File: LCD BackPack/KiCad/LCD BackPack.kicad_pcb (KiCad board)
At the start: 2 copper layers, 45.7 x 22.9 mm, 6 parts, among them J1 8-pin_female_header_LCD_inter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, J2 Conn_01x01_Female, J3 Conn_01x01_Female, U1 LCD_HD44780

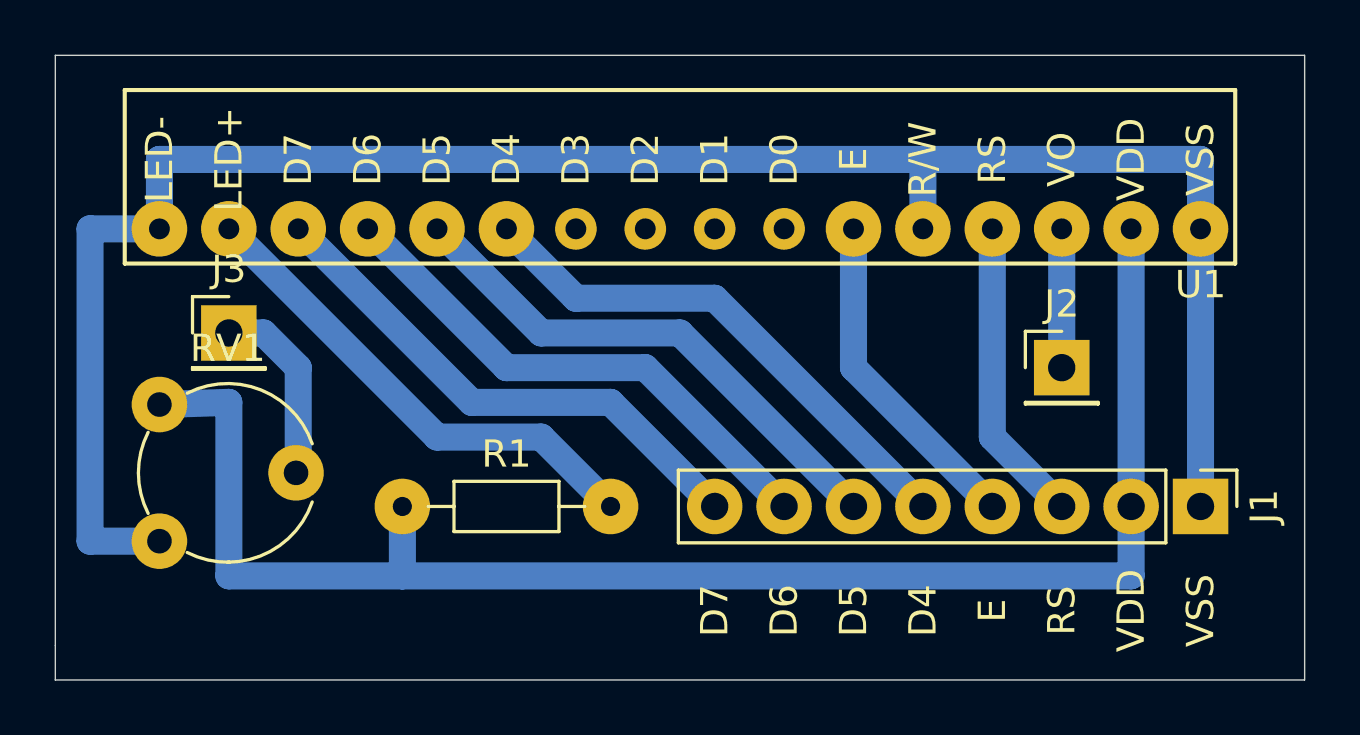
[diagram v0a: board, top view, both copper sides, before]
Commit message: copper pour
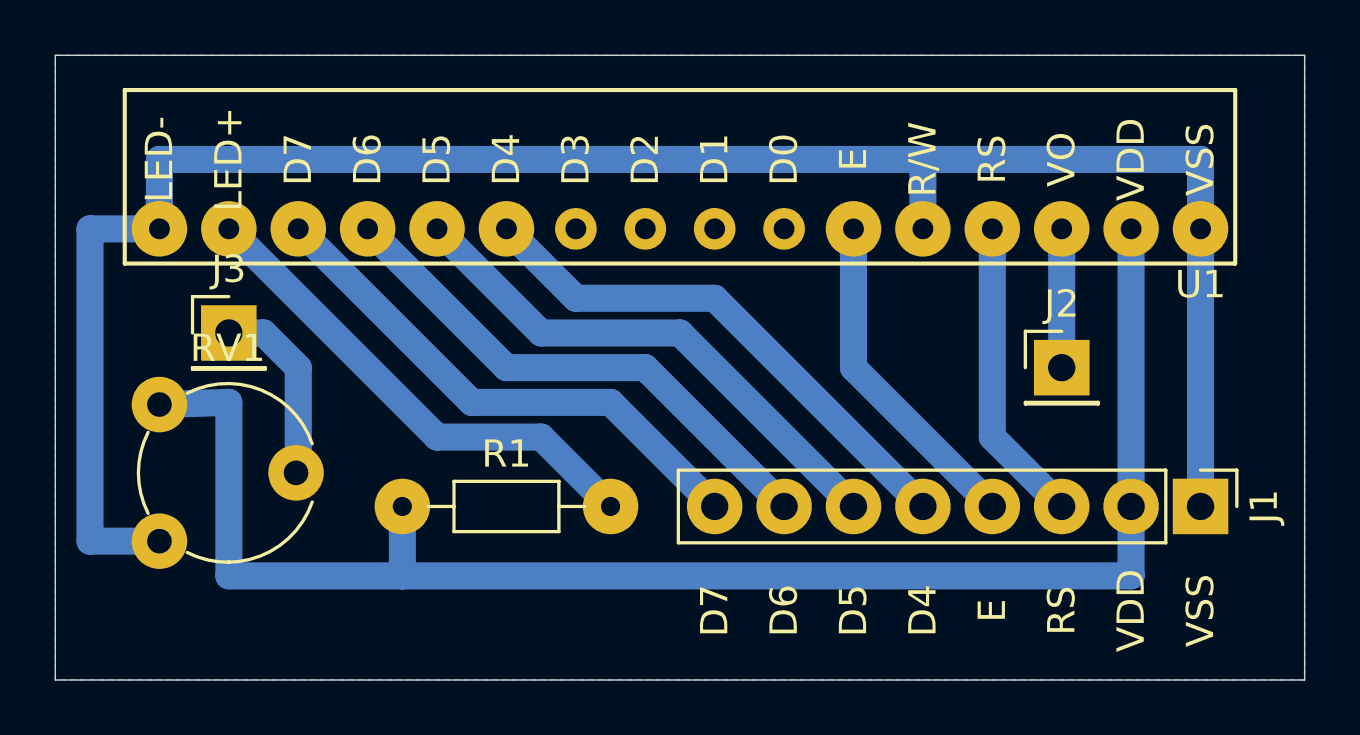
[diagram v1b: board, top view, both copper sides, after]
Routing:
- added copper zone on B.Cu, net Net-(J1-Pad1)
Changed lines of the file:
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@@
   (segment (start 132.08 100.33) (end 133.35 101.6) (width 0.9906) (layer B.Cu) (net 14))
   (segment (start 133.35 101.6) (end 133.35 105.41) (width 0.9906) (layer B.Cu) (net 14))
+  (zone (net 8) (net_name "Net-(J1-Pad1)") (layer B.Cu) (hatch edge 0.508)
+    (connect_pads (clearance 0.508))
+    (min_thickness 0.254)
+    (fill yes (arc_segments 32) (thermal_gap 0.508) (thermal_bridge_width 0.508))
+    (polygon
+      (pts
+        (xy 170.18 113.03) (xy 124.46 113.03) (xy 124.46 90.17) (xy 170.18 90.17)
+      )
+    )
+  )
 )

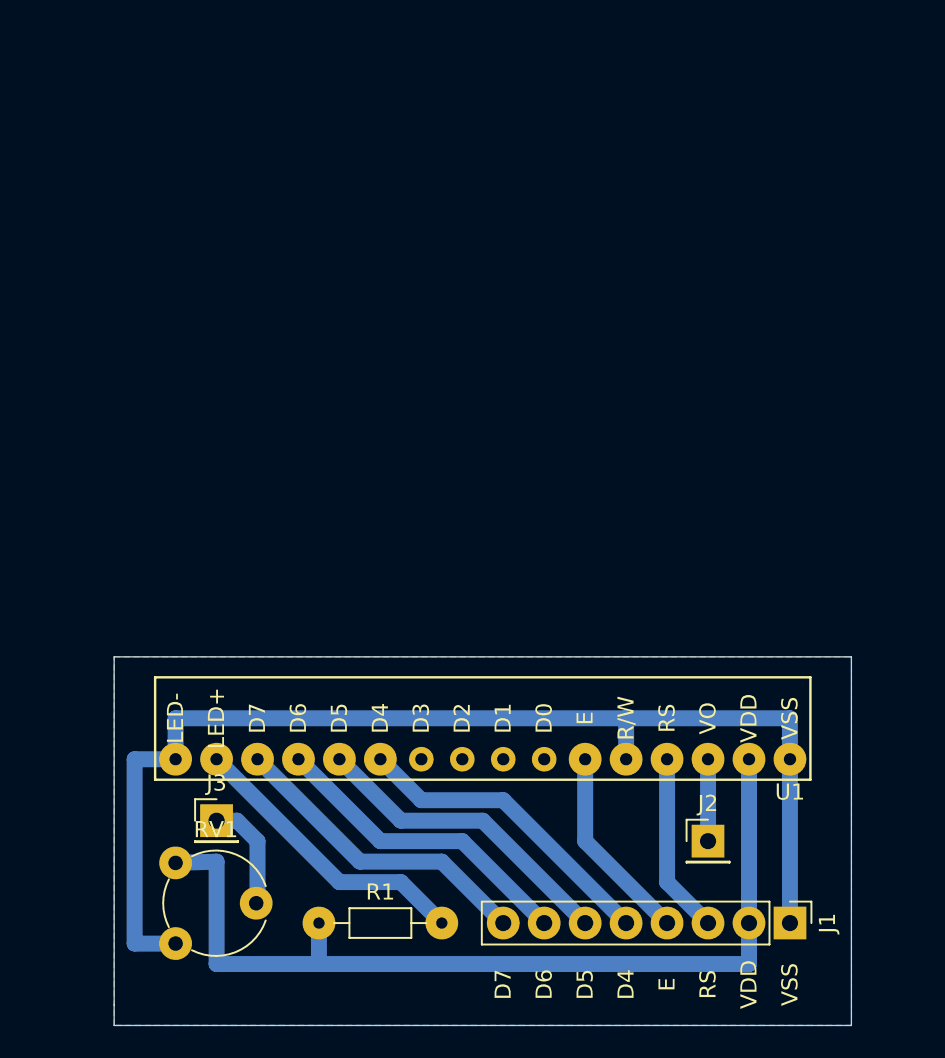
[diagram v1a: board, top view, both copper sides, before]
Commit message: new layout
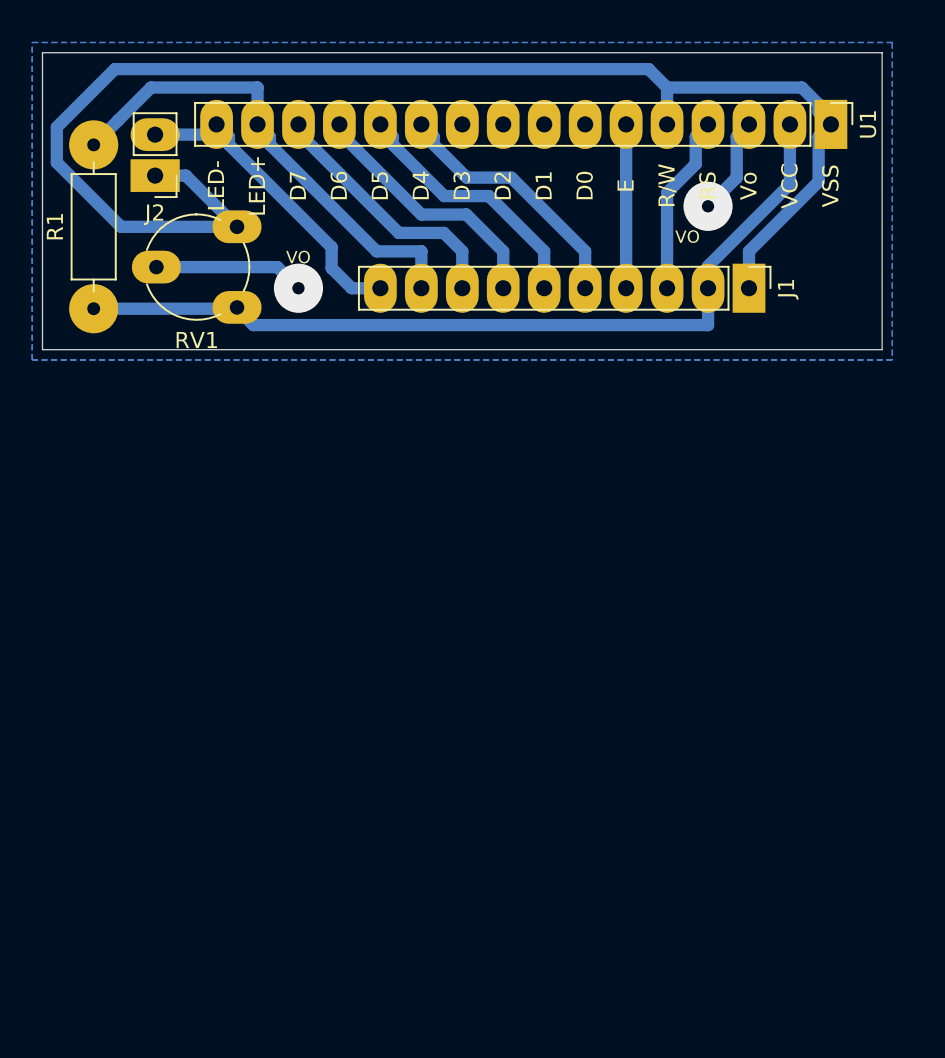
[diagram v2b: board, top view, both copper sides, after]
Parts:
- removed J3: Conn_01x01_Female, Connector_PinHeader_2.54mm:PinHeader_1x01_P2.54mm_Vertical
- J1: value 8-pin_female_header_LCD_interface -> 10-pin_header_LCD_interface; footprint My_Headers:8-pin_LCD_header -> My_Headers:10-pin_LCD_header_larger_pads
- J2: value Conn_01x01_Female -> Conn_01x02_Male; footprint Connector_PinHeader_2.54mm:PinHeader_1x01_P2.54mm_Vertical -> My_Misc:PinHeader_1x02_P2.54mm_Vertical_larger_pads
- R1: footprint Resistor_THT:R_Axial_DIN0204_L3.6mm_D1.6mm_P7.62mm_Horizontal -> My_Misc:R_Axial_DIN0207_L6.3mm_D2.5mm_P10.16mm_Horizontal_larger_pads
- RV1: footprint Potentiometer_THT:Potentiometer_Piher_PT-6-V_Vertical -> My_Misc:Potentiometer_Piher_PT-6-V_Vertical_larger_pads
- U1: footprint My_Headers:16-pin header for LCD HD44780 -> My_Headers:16-pin_LCD_header_larger_pads
- moved J2 53.7 mm to (127.0, 60.3), turned to 180 degrees
- moved RV1 44.6 mm to (132.1, 63.5), turned to 180 degrees
- moved U1 42.0 mm to (168.9, 57.1), turned to 270 degrees
- moved R1 40.6 mm to (123.2, 68.6), turned to 90 degrees
- moved J1 39.5 mm to (163.8, 67.3)
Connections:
- J2 pad 1: Net-(J2-Pad1) -> Net-(J1-Pad1)
- R1 pad 2: Net-(R1-Pad2) -> Net-(J1-Pad9)
- RV1 pad 2: Net-(J2-Pad1) -> Net-(RV1-Pad2)
- U1 pad 10: Net-(U1-Pad10) -> (no net)
- U1 pad 15: Net-(R1-Pad2) -> Net-(J1-Pad9)
- U1 pad 16: Net-(J1-Pad1) -> Net-(J1-Pad10)
- U1 pad 3: Net-(J2-Pad1) -> Net-(RV1-Pad2)
- U1 pad 7: Net-(U1-Pad7) -> (no net)
- U1 pad 8: Net-(U1-Pad8) -> (no net)
- U1 pad 9: Net-(U1-Pad9) -> (no net)
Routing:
- net Net-(J1-Pad9): track 0.00 -> 29.9 mm
- net Net-(J1-Pad10): track 0.00 -> 19.5 mm
- net Net-(R1-Pad2): track 18.2 -> 0.00 mm
- net Net-(RV1-Pad2): track 0.00 -> 15.5 mm, vias 0 -> 2
- net Net-(J1-Pad1): track 72.4 -> 87.2 mm
- net Net-(J2-Pad1): track 12.0 -> 0.00 mm
- net Net-(J1-Pad2): track 57.2 -> 53.1 mm
- net Net-(J1-Pad5): track 19.4 -> 16.0 mm
- net Net-(J1-Pad6): track 19.4 -> 16.0 mm
- net Net-(J1-Pad7): track 19.4 -> 16.0 mm
- net Net-(J1-Pad8): track 19.4 -> 16.0 mm
- net Net-(J1-Pad4): track 12.3 -> 10.2 mm
- added copper zone on B.Cu, net (none)
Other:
- board size 45.7 x 22.9 mm -> 52.1 x 18.4 mm
- net class 30 mil track added: clearance 0.381, trace_width 0.762, via_dia 3.048, via_drill 0.762
- net class 39 mil track removed
- board text added: "VO"

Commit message: kicad6
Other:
- net class 30 mil track removed
- net class Default removed

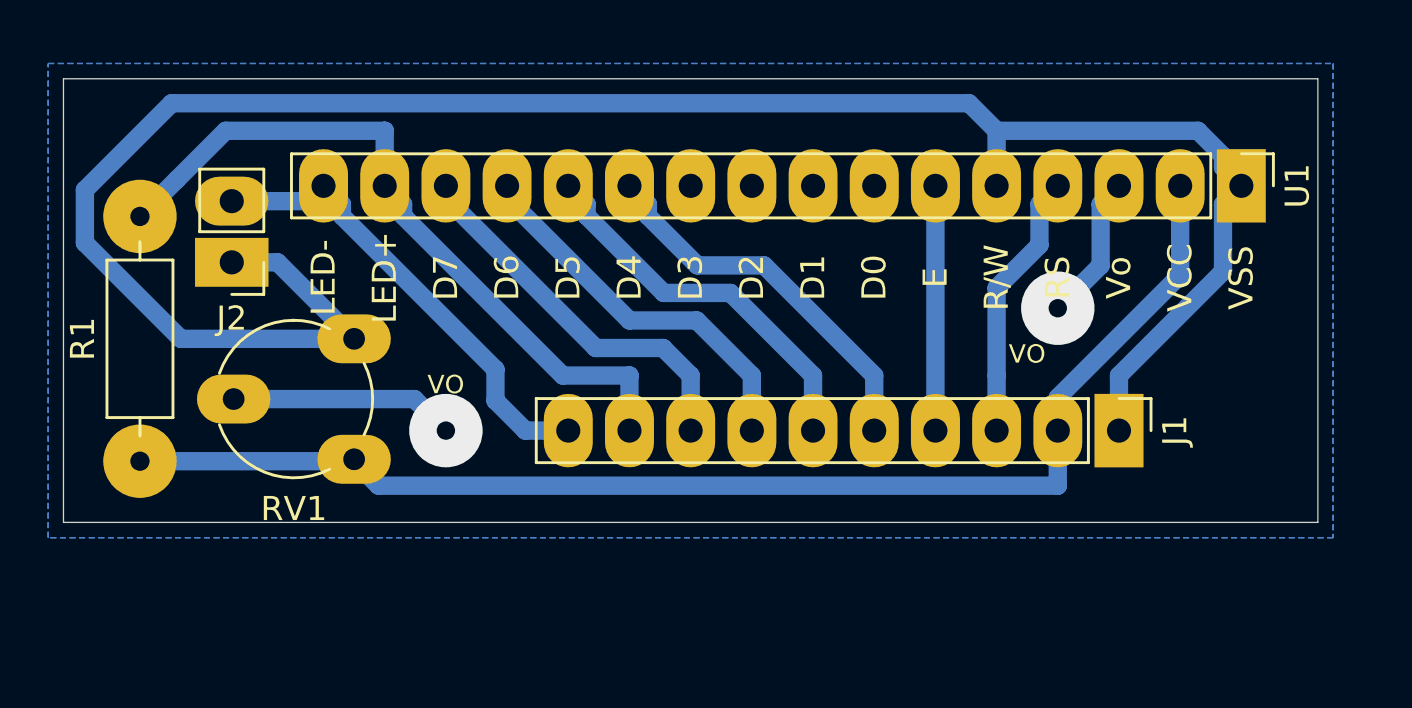
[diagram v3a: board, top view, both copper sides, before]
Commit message: lcd backpack
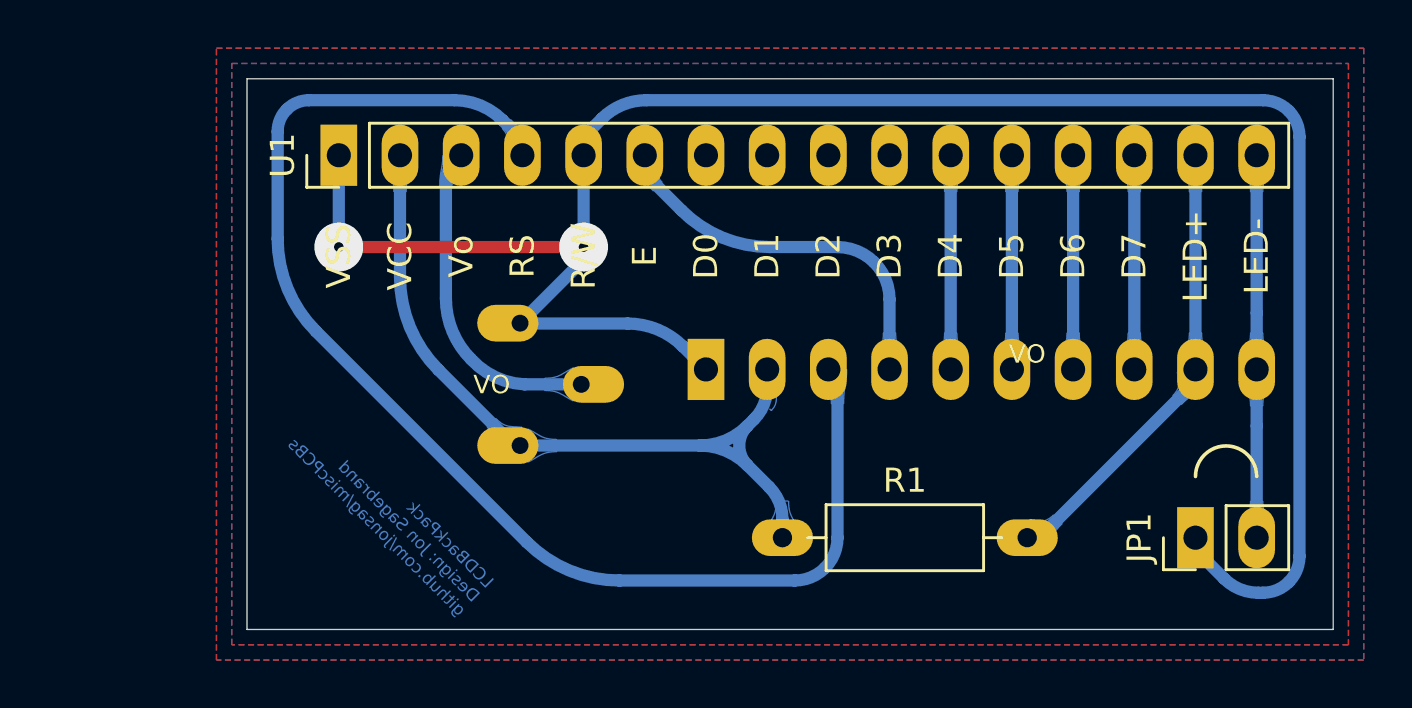
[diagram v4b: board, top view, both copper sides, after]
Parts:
- removed J2: Conn_01x02_Male, My_Misc:PinHeader_1x02_P2.54mm_Vertical_larger_pads
- added JP1: Jumper_2_Open, My_Parts:Angled_Jumper_1x02_P2.54mm_large, F.Cu at (167.0, 71.8)
- J1: moved to B.Cu
- RV1: value 10k -> Contrast; footprint My_Misc:Potentiometer_Piher_PT-6-V_Vertical_larger_pads -> My_Misc:Potentiometer_Bourns_3339P_Vertical_large; moved to B.Cu
- U1: footprint My_Headers:16-pin_LCD_header_larger_pads -> My_Parts:LCD_HD44780_16x2_w_headers_no outlinelarge
- moved U1 37.5 mm to (131.4, 55.9), turned to 0 degrees
- moved R1 26.9 mm to (149.9, 71.8), turned to 0 degrees
- moved J1 17.3 mm to (146.7, 64.8)
- moved RV1 8.19 mm to (139.0, 67.9)
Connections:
- J1 pad 1: Net-(J1-Pad1) -> /GND
- RV1 pad 1: Net-(J1-Pad1) -> Net-(J1-Pad2)
- RV1 pad 3: Net-(J1-Pad2) -> /GND
- U1 pad 1: Net-(J1-Pad1) -> /GND
- U1 pad 10: (no net) -> unconnected-(U1-Pad10)
- U1 pad 5: Net-(J1-Pad1) -> /GND
- U1 pad 7: (no net) -> unconnected-(U1-Pad7)
- U1 pad 8: (no net) -> unconnected-(U1-Pad8)
- U1 pad 9: (no net) -> unconnected-(U1-Pad9)
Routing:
- net Net-(J1-Pad1): track 87.2 -> 0.00 mm
- net /GND: track 0.00 -> 86.4 mm, vias 0 -> 2
- net Net-(J1-Pad3): track 11.2 -> 54.5 mm
- net Net-(J1-Pad2): track 53.1 -> 33.7 mm
- net Net-(J1-Pad9): track 29.9 -> 19.0 mm
- net Net-(J1-Pad8): track 16.0 -> 8.89 mm
- net Net-(J1-Pad7): track 16.0 -> 8.89 mm
- net Net-(J1-Pad5): track 16.0 -> 8.89 mm
- net Net-(J1-Pad6): track 16.0 -> 8.89 mm
- net Net-(J1-Pad4): track 10.2 -> 16.0 mm
- net Net-(J1-Pad10): track 19.5 -> 15.9 mm
- net Net-(U1-Pad3): track 15.5 -> 13.8 mm, vias 2 -> 0
- added copper zone on F.Cu, net (none)
- added copper zone on B.Cu, net /GND
- added copper zone on F.Cu, net /GND
- removed copper zone on B.Cu, net Net-(J1-Pad1)
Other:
- board size 52.1 x 18.4 mm -> 45.1 x 22.9 mm
- board text added: "LCDBackPack Design: Jon Sagebrand github.com/jonsag/miscPCBs"
